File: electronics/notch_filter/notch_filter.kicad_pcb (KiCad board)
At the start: 2 copper layers, 2 parts

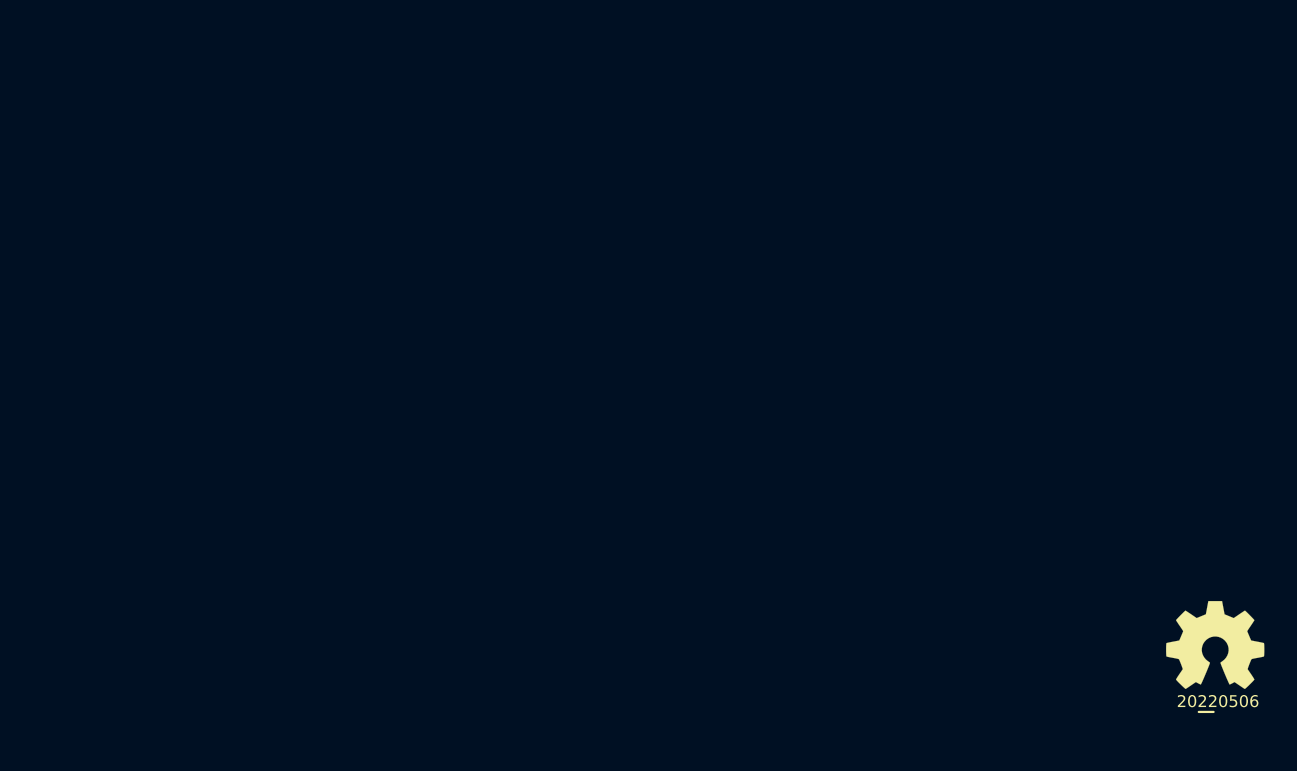
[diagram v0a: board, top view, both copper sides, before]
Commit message: further layout and placing
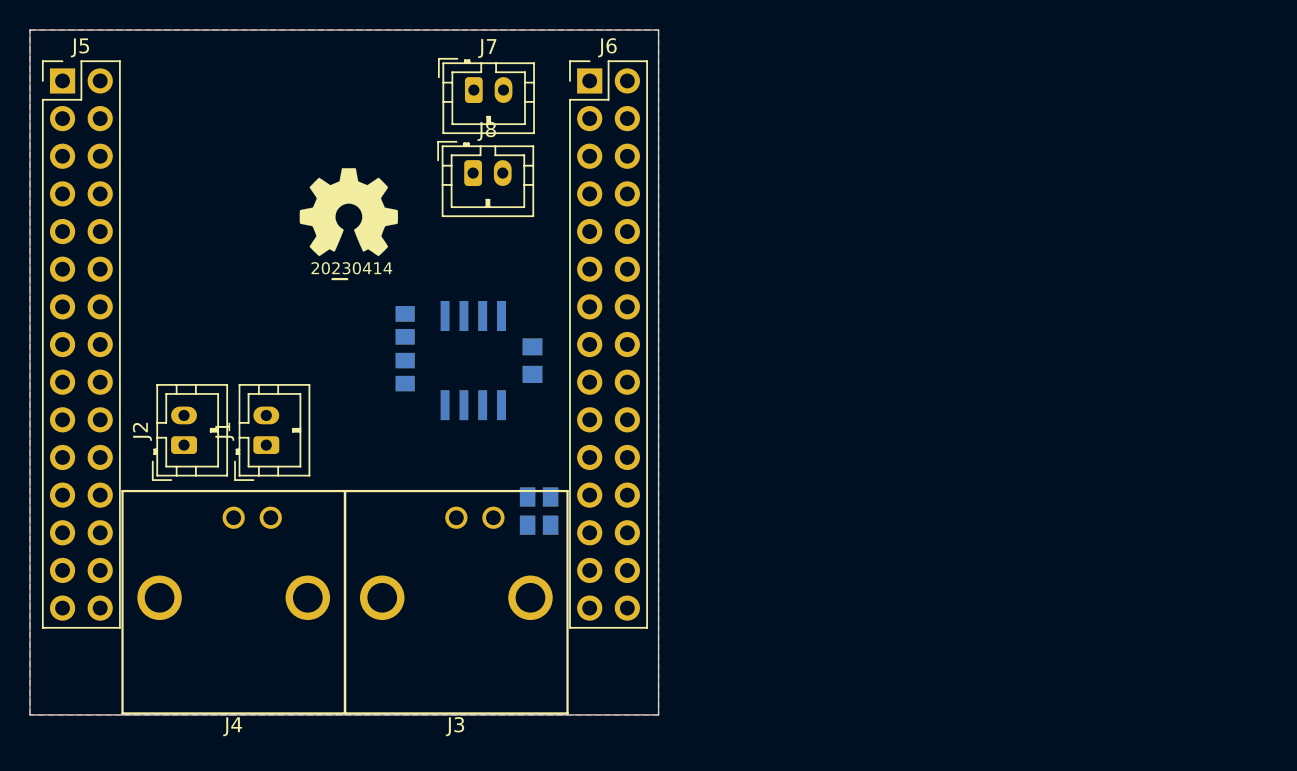
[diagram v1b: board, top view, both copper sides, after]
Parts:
- added C1: 1uF, SquantorRcl:C_0805+0603, B.Cu at (92.7, 68.4)
- added J1: Conn_01x02, Connector_JST:JST_PH_B2B-PH-K_1x02_P2.00mm_Vertical, F.Cu at (74.7, 74.1)
- added J2: Conn_01x02, Connector_JST:JST_PH_B2B-PH-K_1x02_P2.00mm_Vertical, F.Cu at (69.2, 74.1)
- added J3: Output, SquantorConnectors:Conn_BNC_RightAngle_TH, F.Cu at (87.5, 84.4)
- added J4: In, SquantorConnectors:Conn_BNC_RightAngle_TH, F.Cu at (72.5, 84.4)
- added J5: module_2x15_left_input, Connector_PinHeader_2.54mm:PinHeader_2x15_P2.54mm_Vertical, F.Cu at (61.0, 49.5)
- added J6: module_2x15_right_input, Connector_PinHeader_2.54mm:PinHeader_2x15_P2.54mm_Vertical, F.Cu at (96.5, 49.5)
- added J7: Conn_01x02, Connector_JST:JST_PH_B2B-PH-K_1x02_P2.00mm_Vertical, F.Cu at (88.7, 50.1)
- added J8: Conn_01x02, Connector_JST:JST_PH_B2B-PH-K_1x02_P2.00mm_Vertical, F.Cu at (88.7, 55.8)
- added R1: 10K, SquantorRcl:R_0805+0603, B.Cu at (84.1, 66.0)
- added R2: 10K, SquantorRcl:R_0805+0603, B.Cu at (84.1, 69.2)
- added R3: 1.2K, SquantorRcl:R_0805+0603, B.Cu at (93.1, 79.5)
- added R4: 1.2K, SquantorRcl:R_0805+0603, B.Cu at (93.1, 77.6)
- added U1: opamp_single_8pin, SquantorIC:SOIC-8-HAND, B.Cu at (88.7, 68.4)
- N1: value 20220506 -> 20230414
- moved N1 65.3 mm to (79.7, 62.3)
- moved N2 65.3 mm to (80.3, 58.4)
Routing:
- added copper zone on B.Cu, net GND
- added copper zone on F.Cu, net GND
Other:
- board outline added: 42.4 x 46.2 mm
